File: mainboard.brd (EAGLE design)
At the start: 104.8 x 57.1 mm, 16 parts, among them IC1 7805TV, IC2 7805TV, IC3 7805TV, X1 22-23-2021

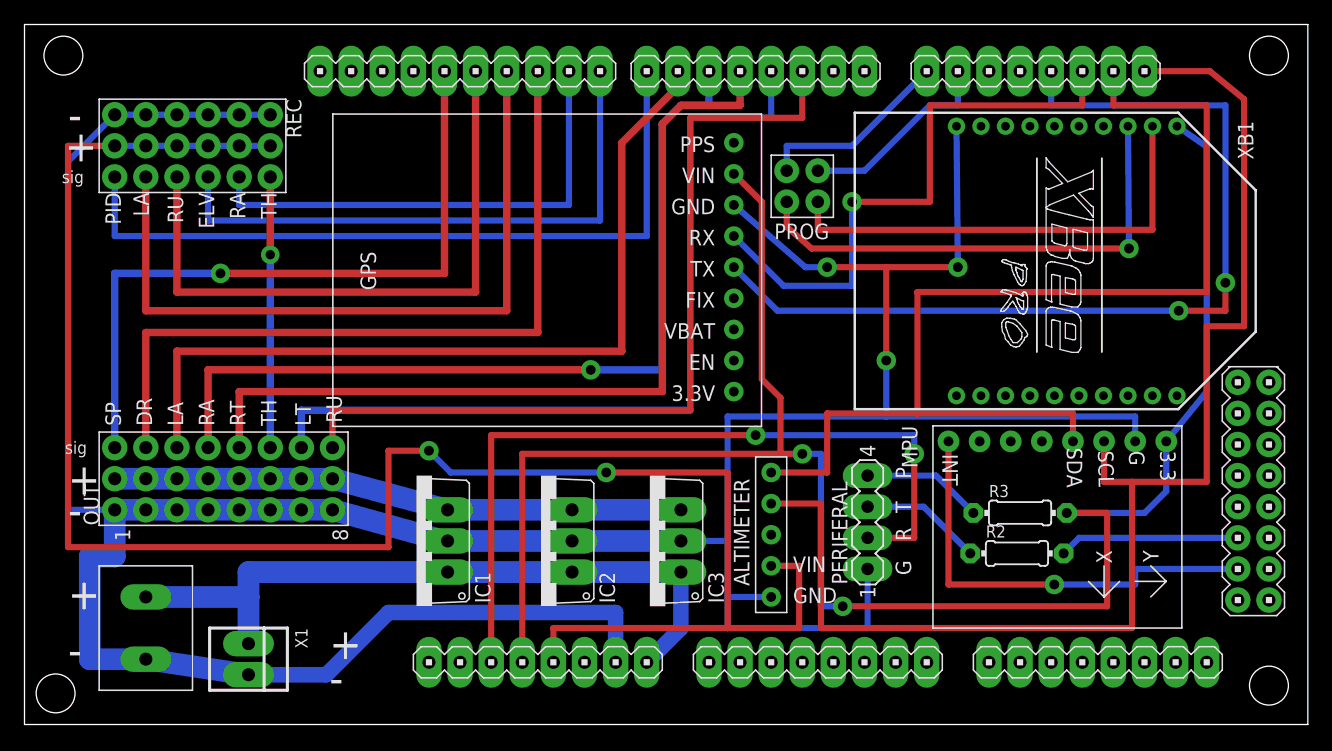
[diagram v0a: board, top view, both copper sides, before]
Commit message: Add files via upload
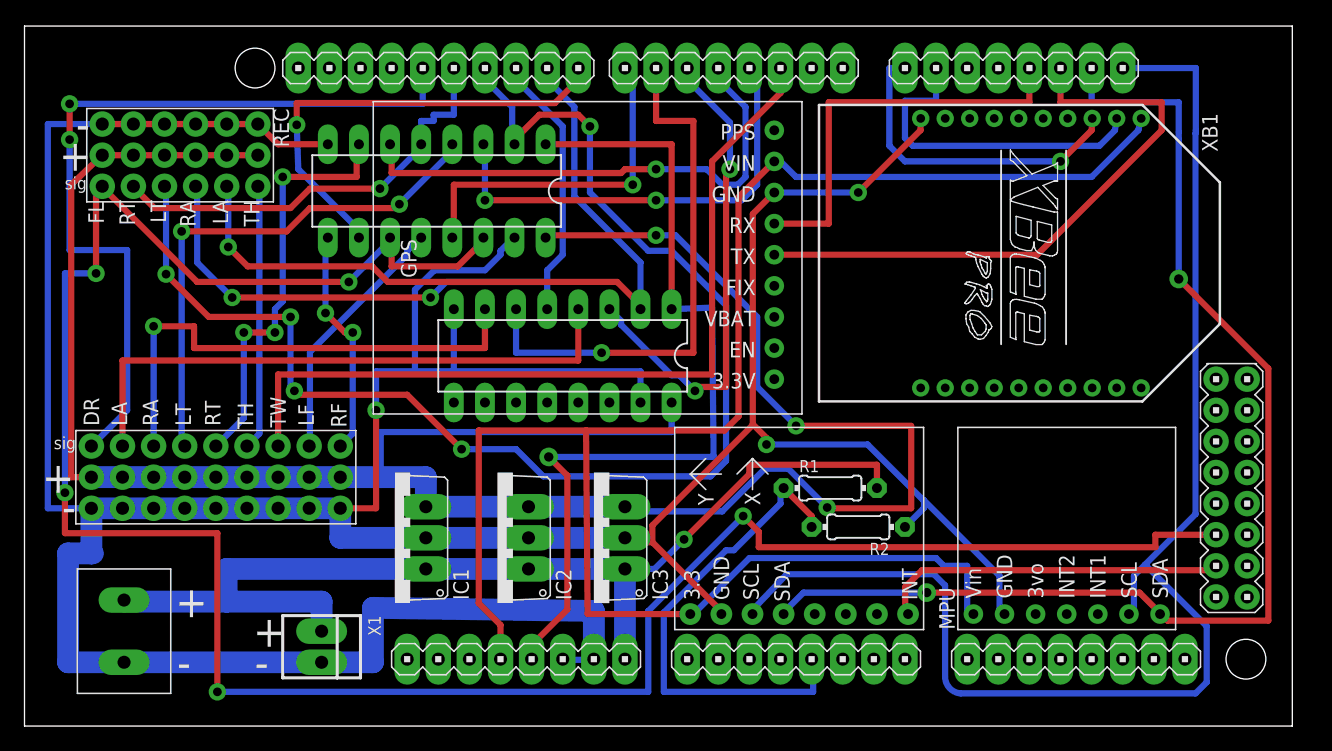
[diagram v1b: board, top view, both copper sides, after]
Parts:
- removed PERIFERAL: (no value), con-lstb:MA04-1
- removed R3: 120, rcl:0204/7
- removed U$2: PIN_2X2, DUElib130425:PIN_2X2
- removed V4: ALTIMETER_V4, aero_sensors:ALTIMETER_V4
- added MUX1, MUX2: SN74HC157, QADT:SN74HC157
- added R1: 100k, rcl:0204/7
- added U$4: ALTIMETER_V5, aero_sensors:ALTIMETER_V5
- G1: device aero_sensors:GPS_ADAFRUIT -> QADT:GPS_ADAFRUIT
- OUT: value PIN_3X8 -> PIN_3X9; device aero_sensors:PIN_3X8 -> QADT:PIN_3X9
- R2: value 120 -> 30k
- moved MPU 21.2 mm to (65.8, 23.0), turned to 90 degrees
- moved R2 13.1 mm to (68.1, 16.1), turned to 180 degrees
- moved X1 6.05 mm to (24.3, 6.35)
- moved IC3 4.58 mm to (46.5, 15.2)
- moved IC2 3.57 mm to (38.6, 15.2)
- moved G1 3.45 mm to (46.0, 38.4)
- moved XB1 2.99 mm to (82.2, 38.5)
- moved OUT 1.91 mm to (13.1, 17.7)
- moved U$1 1.80 mm to (78.2, 23.1)
- moved U$3 1.80 mm to (8.13, 5.08)
- moved IC1 1.80 mm to (30.2, 15.2)
- moved REC 1.27 mm to (14.0, 49.0)
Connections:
- removed net FLAP_MODE: REC.3.5, U$1.11
- removed net LED_ON: PERIFERAL.4, R3.1
- removed net LED_TEST: R2.2, U$1.50
- removed net LED_TEST_OUT: PERIFERAL.3, R2.1
- removed net LEFT_TAIL: OUT.3.7, U$1.3
- removed net N$1: U$1.GND_1
- removed net N$3: U$2.1.1, XB1.3
- removed net N$4: U$2.1.2, XB1.2
- removed net PID_MODE: REC.3.6, U$1.7
- removed net PITCH_R: REC.3.3, U$1.8
- removed net RIGHT_TAIL: OUT.3.5, U$1.4
- removed net ROLL_R: REC.3.2, U$1.9
- removed net RUDDER: OUT.3.8, U$1.2
- removed net RX1: G1.RX, U$1.RX1
- removed net SPARE: OUT.3.1, U$1.13
- removed net TX1: G1.TX, U$1.TX1
- removed net YAW_R: REC.3.4, U$1.12
- new net BATTERY_VOLTAGE_IN: R1.1, R2.2, U$1.A4
- new net DUE-TO-GPS: G1.RX, U$1.TX1
- new net FLAPS_IN: MUX2.11, MUX2.14, REC.3.6, U$1.50
- new net FLAPS_LEFT: MUX2.12, OUT.3.8
- new net FLAPS_LEFT_AOUT: MUX2.13, U$1.7
- new net FLAPS_RIGHT: MUX2.9, OUT.3.9
- new net FLAPS_RIGHT_AOUT: MUX2.10, U$1.8
- new net GPS-TO-DUE: G1.TX, U$1.RX1
- new net LEFT_AILERON_AOUT: MUX1.3, U$1.5
- new net LEFT_AILERON_IN: MUX1.2, REC.3.2, U$1.9
- new net LEFT_VTAIL: MUX2.4, OUT.3.4
- new net LEFT_VTAIL_AOUT: MUX2.3, U$1.3
- new net LEFT_VTAIL_IN: MUX2.2, REC.3.4, U$1.11
- new net RIGHT_AILERON_AOUT: MUX1.6, U$1.6
- new net RIGHT_AILERON_IN: MUX1.5, REC.3.3, U$1.10
- new net RIGHT_VTAIL: MUX2.7, OUT.3.5
- new net RIGHT_VTAIL_AOUT: MUX2.6, U$1.4
- new net RIGHT_VTAIL_IN: MUX2.5, REC.3.5, U$1.12
- new net TAIL_WHEEL: OUT.3.7, U$1.2
- net +5V: now also MUX1.1, MUX2.1; no longer REC.2.1, REC.2.2, REC.2.3, REC.2.4, REC.2.5, REC.2.6, V4.VIN
- net 12V: now also R1.2
- net 3.3V: now also U$4.VIN; no longer R3.2
- net DROP: now also OUT.3.1, U$1.13; no longer OUT.3.2, U$1.10
- net GND: now also MUX1.15, MUX1.8, MUX2.15, MUX2.8, OUT.1.9, R2.1, U$1.GND_1, U$4.GND; no longer PERIFERAL.1, V4.GND
- net LEFT_AILERON: now also MUX1.4, OUT.3.2; no longer OUT.3.3, U$1.6
- net RESET: no longer PERIFERAL.2
- net RIGHT_AILERON: now also MUX1.7, OUT.3.3; no longer OUT.3.4, U$1.5
- net RX: now also XB1.2; no longer U$2.2.2
- net SCL: now also U$4.SCL; no longer V4.SCL
- net SDA: now also U$4.SDA; no longer V4.SDA
- net SERVO_PWR: now also MUX1.16, MUX2.16, OUT.2.9, REC.2.1, REC.2.2, REC.2.3, REC.2.4, REC.2.5, REC.2.6
- net TX: now also XB1.3; no longer U$2.2.1
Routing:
- net FLAPS_IN: track 0.00 -> 190.6 mm, vias 0 -> 5
- net SERVO_PWR: track 46.6 -> 190.3 mm, vias 0 -> 3
- net LEFT_VTAIL_IN: track 0.00 -> 111.8 mm, vias 0 -> 5
- net +5V: track 154.7 -> 71.1 mm, vias 2 -> 1
- net TX1: track 75.4 -> 0.00 mm, vias 2 -> 0
- net RIGHT_TAIL: track 70.7 -> 0.00 mm
- net LEFT_TAIL: track 69.1 -> 0.00 mm
- net RUDDER: track 69.1 -> 0.00 mm
- net TAIL_WHEEL: track 0.00 -> 68.6 mm
- net RESET: track 65.3 -> 0.00 mm, vias 2 -> 0
- net LEFT_AILERON_IN: track 0.00 -> 63.8 mm, vias 0 -> 1
- net PID_MODE: track 61.7 -> 0.00 mm
- net FLAP_MODE: track 59.9 -> 0.00 mm
- net RIGHT_AILERON_IN: track 0.00 -> 58.3 mm, vias 0 -> 2
- net SPARE: track 57.7 -> 0.00 mm, vias 1 -> 0
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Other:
- board size 104.8 x 57.1 mm -> 103.5 x 57.2 mm
- board text added: "FL"
- board text added: "GND"
- board text added: "LF"
- board text added: "RF"
- board text added: "TW"
- board text removed: "ELV"
- board text removed: "G"
- board text removed: "P"
- board text removed: "PID"
- board text removed: "PROG"
- board text removed: "R"
- board text removed: "RU"
- board text removed: "SP"
- board text removed: "T"
